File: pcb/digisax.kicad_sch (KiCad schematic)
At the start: 53 parts, among them SW1 RotaryEncoder_Switch, U1 ER_OLEDM0.91_1x-I2C, U2 MPXV7007, U3 MCP3221, U4 TLV320DAC3100_breakout, U5 ESP32-S3

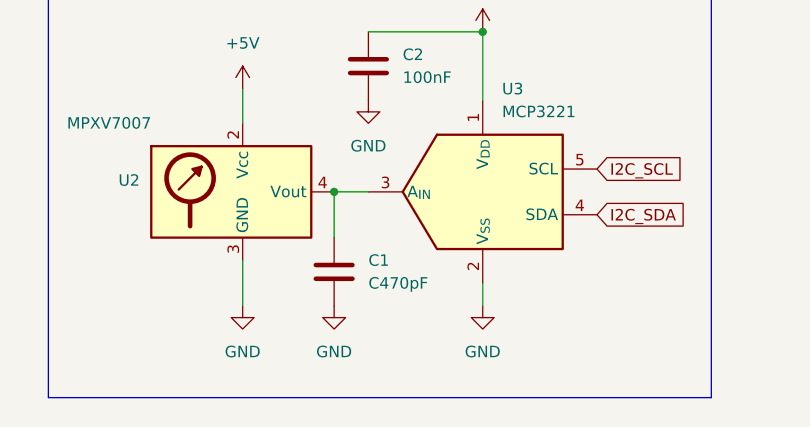
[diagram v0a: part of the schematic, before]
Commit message: added all symbols :D
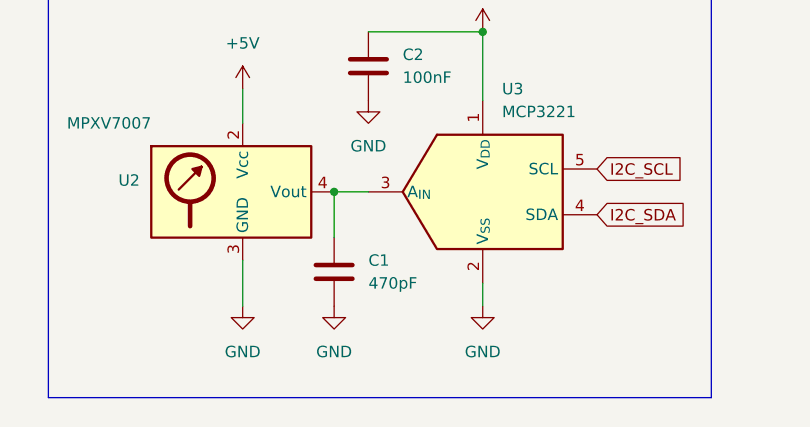
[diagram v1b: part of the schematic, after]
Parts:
- BT1: footprint (none) -> digisax_stuff:5V0_terminal
- C1: value C470pF -> 470pF; footprint (none) -> Capacitor_THT:C_Disc_D4.7mm_W2.5mm_P5.00mm
- C2, C3: footprint (none) -> Capacitor_THT:C_Disc_D4.7mm_W2.5mm_P5.00mm
- C4: footprint (none) -> Capacitor_THT:CP_Radial_D6.3mm_P2.50mm
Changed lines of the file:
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@@
 			)
 		)
-		(property "Footprint" ""
+		(property "Footprint" "Capacitor_THT:C_Disc_D4.7mm_W2.5mm_P5.00mm"
 			(at 133.0452 151.13 0)
 			(hide yes)
@@
 			)
 		)
-		(property "Value" "C470pF"
+		(property "Value" "470pF"
 			(at 132.08 171.4499 0)
 			(show_name no)
@@
 			)
 		)
-		(property "Footprint" ""
+		(property "Footprint" "Capacitor_THT:C_Disc_D4.7mm_W2.5mm_P5.00mm"
 			(at 129.2352 173.99 0)
 			(hide yes)
@@
 			)
 		)
-		(property "Footprint" ""
+		(property "Footprint" "digisax_stuff:5V0_terminal"
 			(at 187.96 97.536 90)
 			(hide yes)
@@
 			)
 		)
-		(property "Footprint" ""
+		(property "Footprint" "Capacitor_THT:C_Disc_D4.7mm_W2.5mm_P5.00mm"
 			(at 188.9252 74.93 0)
 			(hide yes)
@@
 			)
 		)
-		(property "Footprint" ""
+		(property "Footprint" "Capacitor_THT:CP_Radial_D6.3mm_P2.50mm"
 			(at 202.8952 102.87 0)
 			(hide yes)
